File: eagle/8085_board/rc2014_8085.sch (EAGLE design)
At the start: 17 parts, among them IC1 74HCT14N, IC3 74HCT573N

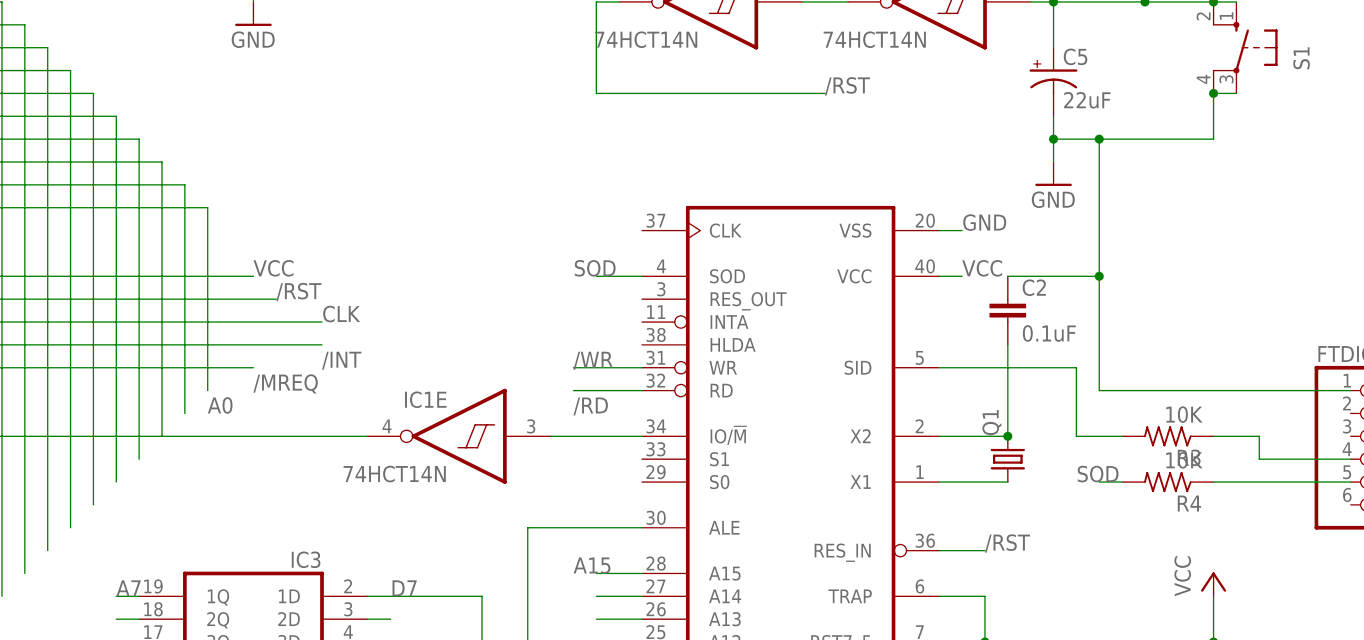
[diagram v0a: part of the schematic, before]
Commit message: Clean up, add CLK
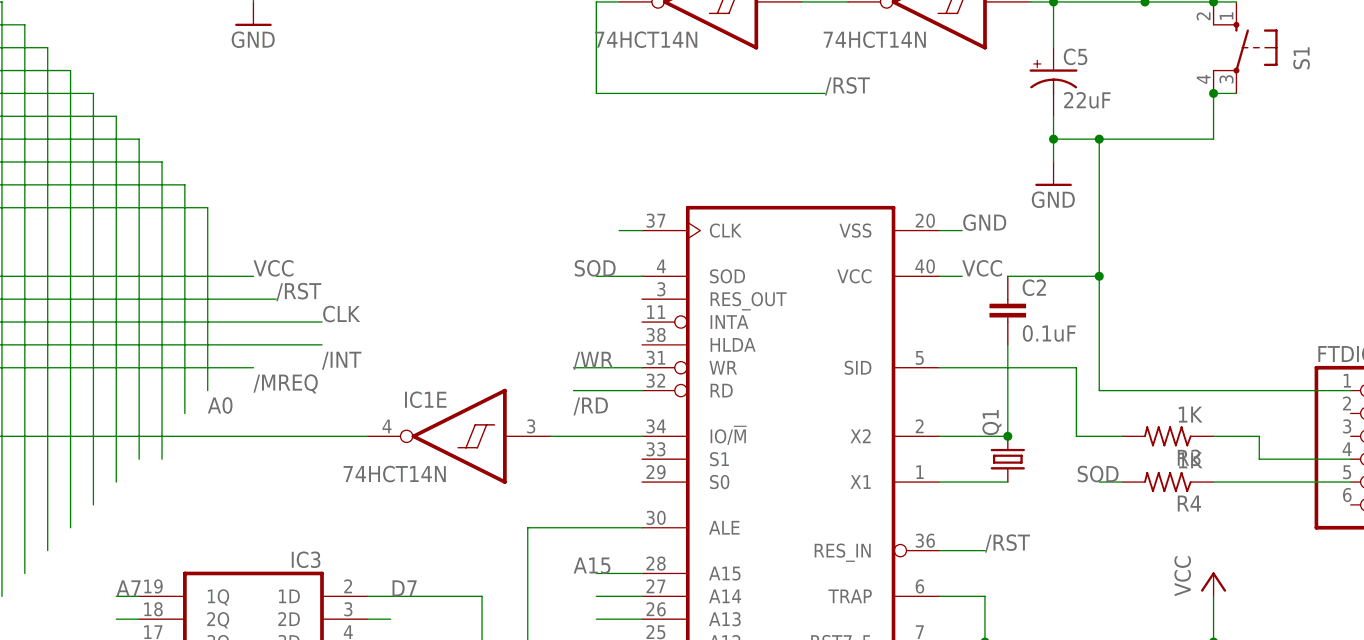
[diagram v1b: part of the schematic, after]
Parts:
- R3, R4: value 10K -> 1K
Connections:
- net N$2 renamed ALE
- net N$3 renamed TX
- net N$4 renamed RX
- net CLK: now also IC2.CLK
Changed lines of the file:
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@@
 <?xml version="1.0" encoding="utf-8"?>
 <!DOCTYPE eagle SYSTEM "eagle.dtd">
-<eagle version="8.1.0">
+<eagle version="8.1.1">
 <drawing>
 <settings>
@@
 <part name="C2" library="rcl" deviceset="C-EU" device="050-024X044" value="0.1uF"/>
 <part name="R2" library="rcl" deviceset="R-US_" device="0207/10" value="10K"/>
-<part name="R3" library="rcl" deviceset="R-US_" device="0207/10" value="10K"/>
-<part name="R4" library="rcl" deviceset="R-US_" device="0207/10" value="10K"/>
+<part name="R3" library="rcl" deviceset="R-US_" device="0207/10" value="1K"/>
+<part name="R4" library="rcl" deviceset="R-US_" device="0207/10" value="1K"/>
 </parts>
 <sheets>
@@
 <pinref part="_PIN1" gate="-1" pin="14"/>
 <wire x1="-104.14" y1="149.86" x2="-35.56" y2="149.86" width="0.1524" layer="91"/>
-<wire x1="-35.56" y1="119.38" x2="-35.56" y2="149.86" width="0.1524" layer="91"/>
+<wire x1="-35.56" y1="116.84" x2="-35.56" y2="149.86" width="0.1524" layer="91"/>
 </segment>
 <segment>
@@
 <label x="-17.78" y="132.08" size="1.778" layer="95"/>
 </segment>
+<segment>
+<pinref part="IC2" gate="G$1" pin="CLK"/>
+<wire x1="17.78" y1="142.24" x2="15.24" y2="142.24" width="0.1524" layer="91"/>
+</segment>
 </net>
 <net name="/MREQ" class="0">
@@
 </segment>
 </net>
-<net name="N$2" class="0">
+<net name="ALE" class="0">
 <segment>
 <pinref part="IC3" gate="A" pin="C"/>
@@
 </segment>
 </net>
-<net name="N$3" class="0">
+<net name="TX" class="0">
 <segment>
 <pinref part="R4" gate="G$1" pin="1"/>
@@
 </segment>
 </net>
-<net name="N$4" class="0">
+<net name="RX" class="0">
 <segment>
 <pinref part="R3" gate="G$1" pin="1"/>
@@
 </sheet>
 </sheets>
+<errors>
+</errors>
 </schematic>
 </drawing>
